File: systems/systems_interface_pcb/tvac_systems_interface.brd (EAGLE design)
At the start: 137.1 x 100 mm, 6 parts, among them J1 171-025-213R001, J2 A-DS09A/KG-T2S, J3 A-DS09A/KG-T2S, J4 A-DS09A/KG-T2S, X1 TERMINAL-BLOCK-3.5MM-6-PIN-RO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

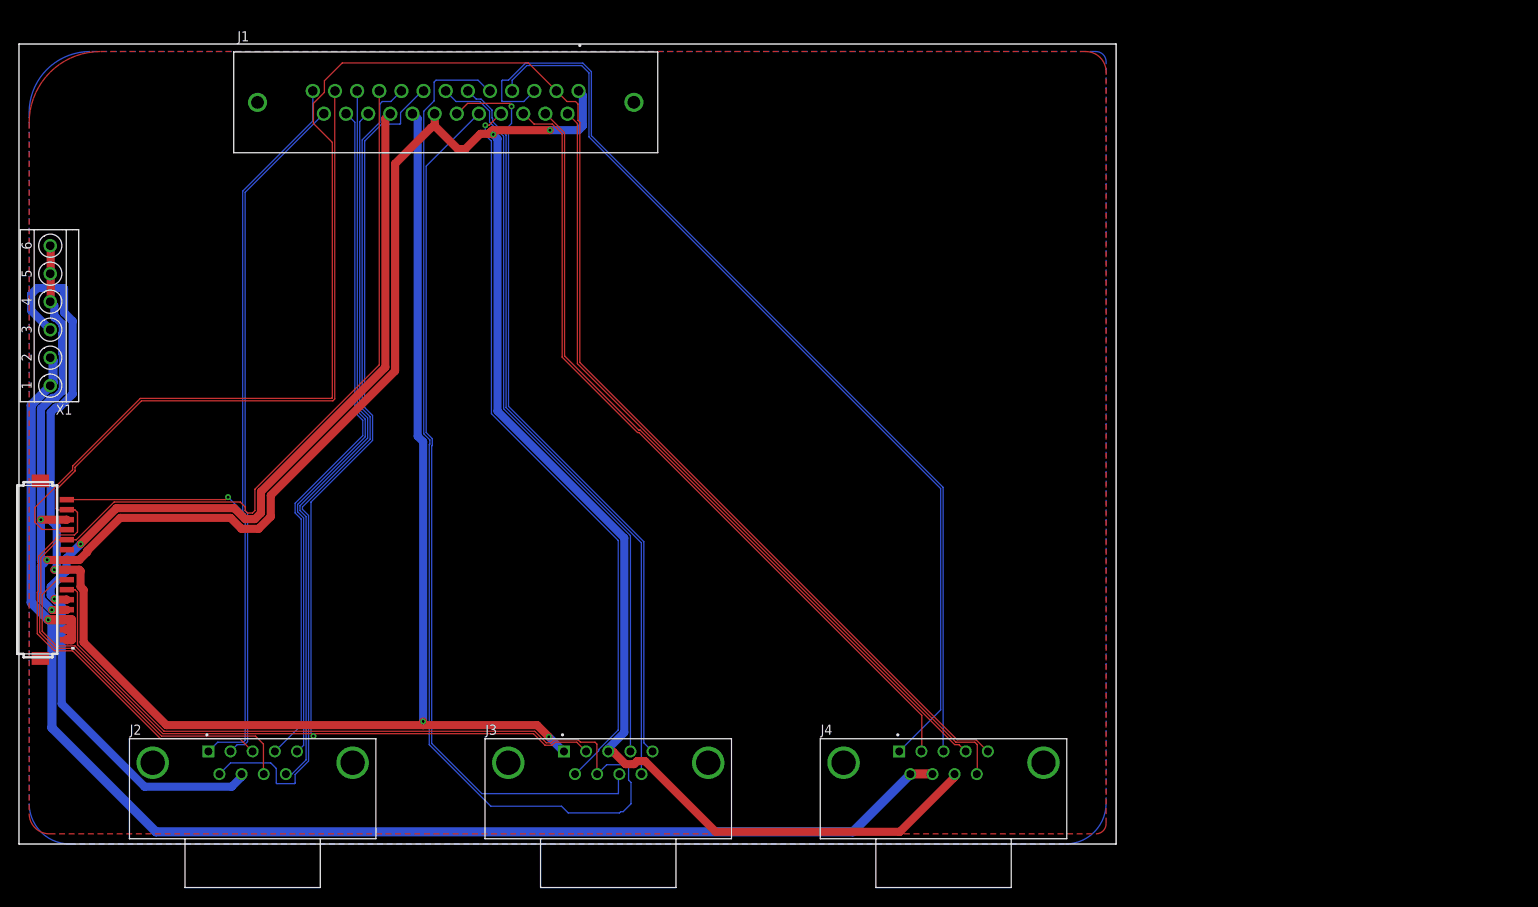
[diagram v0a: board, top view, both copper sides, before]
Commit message: Add files via upload
hand-routed using Jaden and Lorna's advice
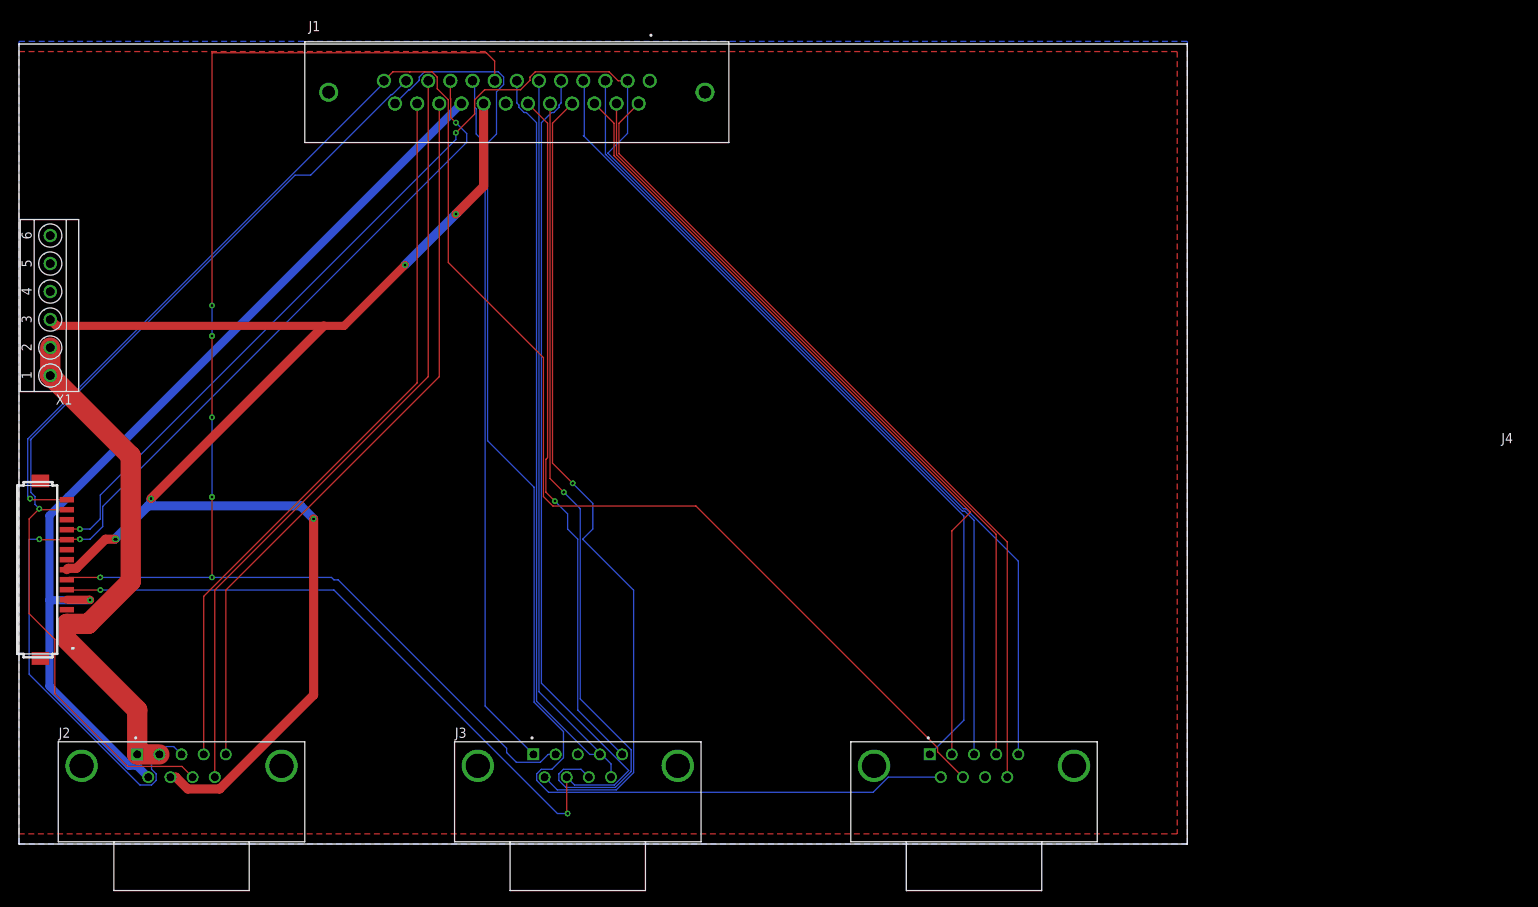
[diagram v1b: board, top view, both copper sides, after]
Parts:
- moved J1 8.98 mm to (62.2, 94.0)
- moved J2 8.90 mm to (20.3, 9.78)
- moved J3 3.83 mm to (69.8, 9.78)
- moved J4 3.83 mm to (119.4, 9.78)
- moved X1 1.27 mm to (3.81, 67.3)
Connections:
- net +3V3: now also J2.8; no longer J3.1
- net +5V: now also J2.9; no longer J2.8
- net +BAT: now also J2.1, J2.2; no longer J4.8, J4.9
- net CANH: now also J2.7; no longer J2.3
- net CANL: now also J4.8; no longer J2.1
- net DIS_TRANS_UARTN: now also J2.5; no longer J2.6
- net PAY_MOSI_A/TX: now also J3.1; no longer J2.9
- net PAY_RST: now also J2.6; no longer J2.5
- net PAY_SCK_A/TX: now also J2.3; no longer J2.7
- net RTC_VBATT: now also J4.9; no longer J2.2
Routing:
- net GND: track 306.6 -> 0.00 mm, vias 5 -> 0
- net +BAT: track 173.7 -> 65.1 mm, vias 1 -> 0
- net CANL: track 113.0 -> 208.3 mm
- net RTC_VBATT: track 85.3 -> 162.5 mm
- net EPS_RST: track 212.1 -> 179.6 mm, vias 0 -> 2
- net MISO_A: track 228.8 -> 204.4 mm, vias 0 -> 2
- net EPS_MOSI_A/TX: track 122.9 -> 103.5 mm
- net PAY_MOSI_A/TX: track 106.3 -> 87.4 mm
- net +3V3: track 202.4 -> 185.7 mm, vias 3 -> 6
- net +5V: track 133.2 -> 119.2 mm, vias 2 -> 1
- net EPS_SCK_A/TX: track 117.3 -> 105.9 mm
- net PAY_RST: track 87.2 -> 98.1 mm
- net CANH: track 135.0 -> 124.7 mm, vias 0 -> 1
- net D_GATE: track 92.8 -> 102.6 mm
- net RELEASE_B: track 96.0 -> 86.4 mm
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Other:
- board size 137.1 x 100 mm -> 146 x 100 mm
- board text removed: "UTAT-SS HERON MKII TVAC SYSTEM INTERFACE PCB"
